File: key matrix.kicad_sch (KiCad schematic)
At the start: 62 parts, among them J3 Conn_01x04_MountingPin, J4 Conn_01x04_MountingPin, SW1 SW_Push, SW10 SW_Push, SW11 SW_Push, SW12 SW_Push, SW13 SW_Push, SW14 SW_Push, SW15 SW_Push, SW16 SW_Push, SW17 SW_Push, SW18 SW_Push, SW19 SW_Push, SW2 SW_Push, SW20 SW_Push, SW21 SW_Push, SW22 SW_Push, SW23 SW_Push, SW24 SW_Push, SW25 SW_Push, SW26 SW_Push, SW27 SW_Push, SW28 SW_Push, SW29 SW_Push, SW3 SW_Push, SW30 SW_Push, SW31 SW_Push, SW32 SW_Push, SW33 SW_Push, SW34 SW_Push, SW35 SW_Push, SW36 SW_Push, SW37 SW_Push, SW38 SW_Push, SW39 SW_Push, SW4 SW_Push, SW40 SW_Push, SW41 SW_Push, SW42 SW_Push, SW43 RotaryEncoder_Switch_MP, SW44 RotaryEncoder_Switch_MP, SW45 SW_Push, SW46 SW_Push, SW47 SW_Push, SW48 SW_Push, SW5 SW_Push, SW6 SW_Push, SW7 SW_Push, SW8 SW_Push, SW9 SW_Push, U1 BAT54CTB6_R1_00001, U10 BAT54CTB6_R1_00001, U11 BAT54CTB6_R1_00001, U12 BAT54CTB6_R1_00001, U2 BAT54CTB6_R1_00001, U3 BAT54CTB6_R1_00001, U4 BAT54CTB6_R1_00001, U5 BAT54CTB6_R1_00001, U6 BAT54CTB6_R1_00001, U7 BAT54CTB6_R1_00001, U8 BAT54CTB6_R1_00001, U9 BAT54CTB6_R1_00001

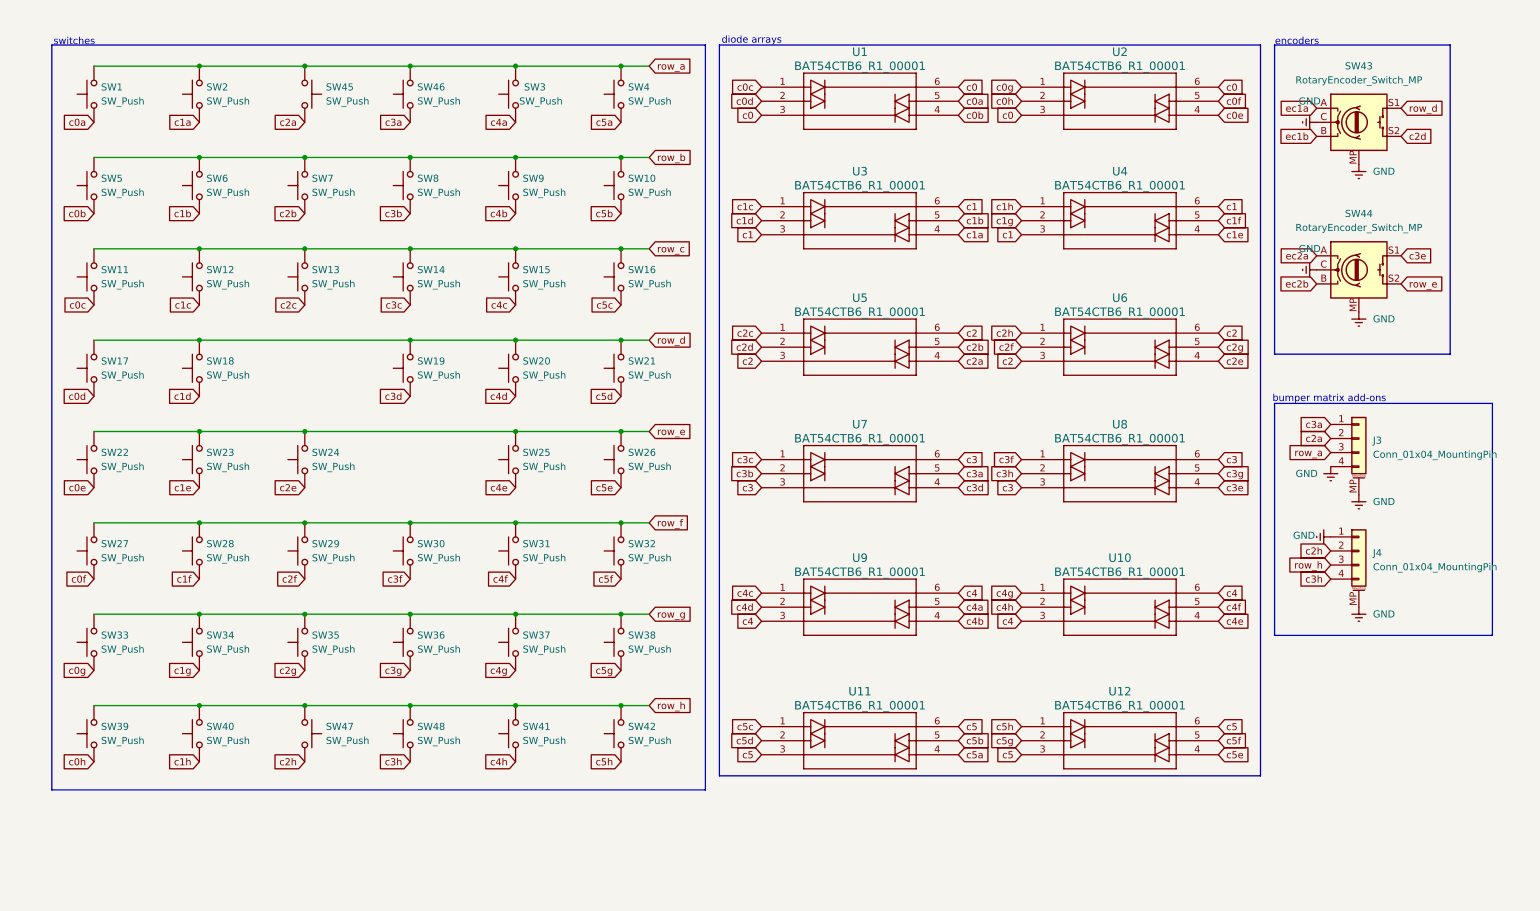
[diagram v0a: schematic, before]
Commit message: parpar v2 RC2
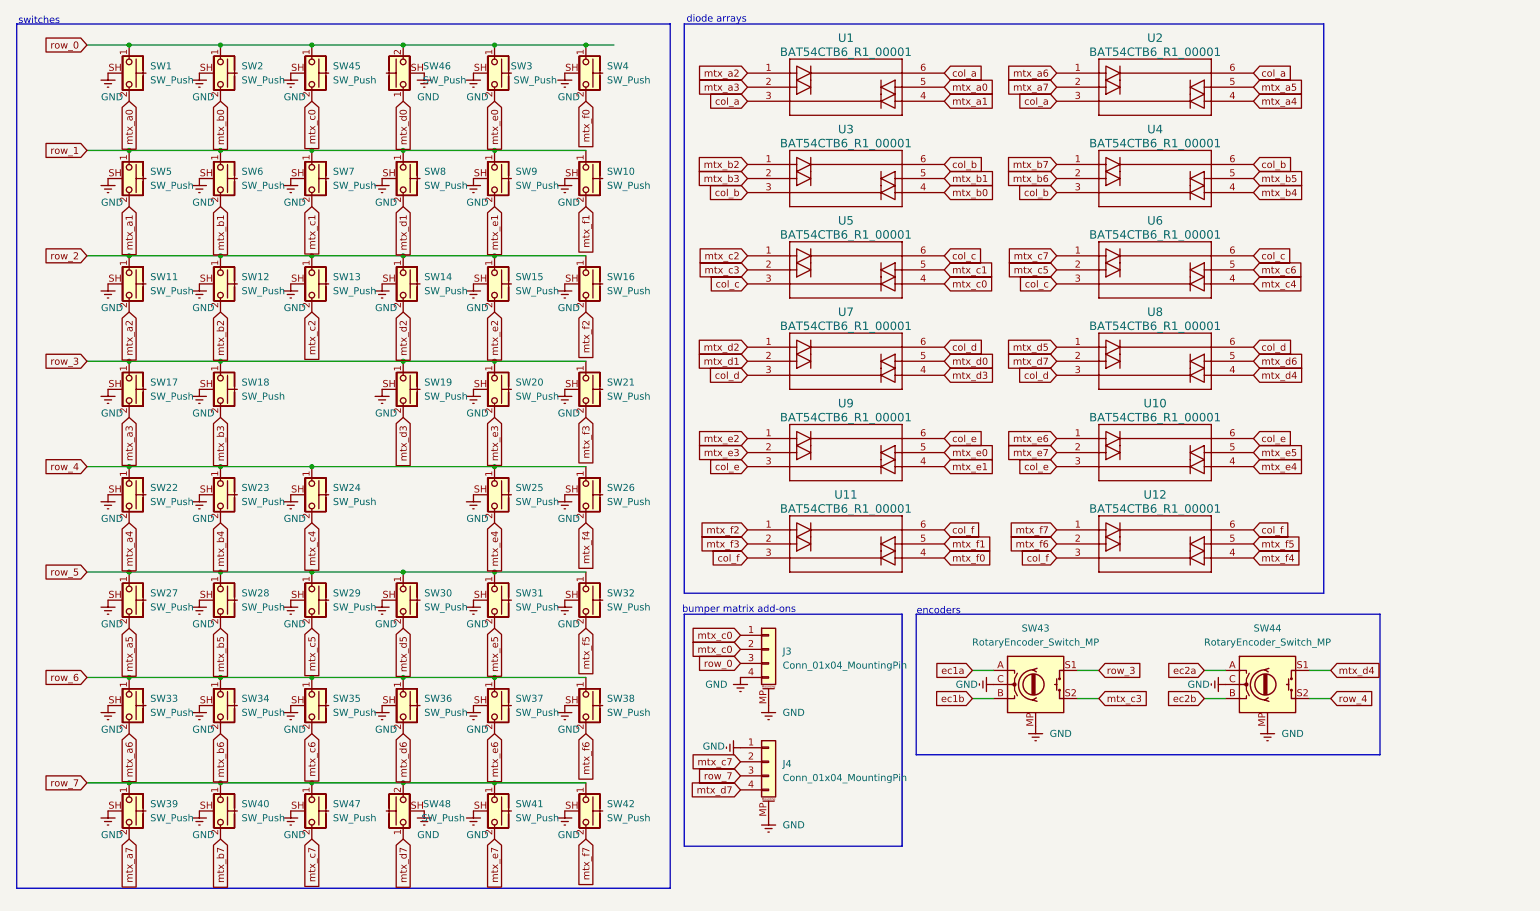
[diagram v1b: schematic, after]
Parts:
- SW1, SW10, SW11, SW12, SW13, SW14, SW15, SW16, SW17, SW18, SW19, SW2, SW20, SW21, SW22, SW23, SW24, SW25, SW26, SW27, SW28, SW29, SW3, SW30, SW31, SW32, SW33, SW34, SW35, SW36, SW37, SW38, SW39, SW4, SW40, SW41, SW42, SW5, SW6, SW7, SW8, SW9: footprint coquette_footprints:choc1u-hs-modded -> coquette_footprints:SW_Hotswap_Kailh_Choc_V1V2_Plated_modded; symbol Switch:SW_Push -> Switch:SW_Push_Shielded
- SW45, SW46, SW47, SW48: symbol Switch:SW_Push -> Switch:SW_Push_Shielded
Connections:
- net GND: now also SW1.SH (B), SW10.SH (B), SW11.SH (B), SW12.SH (B), SW13.SH (B), SW14.SH (B), SW15.SH (B), SW16.SH (B), SW17.SH (B), SW18.SH (B), SW19.SH (B), SW2.SH (B), SW20.SH (B), SW21.SH (B), SW22.SH (B), SW23.SH (B), SW24.SH (B), SW25.SH (B), SW26.SH (B), SW27.SH (B), SW28.SH (B), SW29.SH (B), SW3.SH (B), SW30.SH (B), SW31.SH (B), SW32.SH (B), SW33.SH (B), SW34.SH (B), SW35.SH (B), SW36.SH (B), SW37.SH (B), SW38.SH (B), SW39.SH (B), SW4.SH (B), SW40.SH (B), SW41.SH (B), SW42.SH (B), SW45.SH (B), SW46.SH (B), SW47.SH (B), SW48.SH (B), SW5.SH (B), SW6.SH (B), SW7.SH (B), SW8.SH (B), SW9.SH (B)
- net c0 renamed col_a
- net c0a renamed mtx_a0
- net mtx_a0: now also SW1.2; no longer SW1.1
- net c0b renamed mtx_a1
- net mtx_a1: now also SW5.2; no longer SW5.1
- net c0c renamed mtx_a2
- net mtx_a2: now also SW11.2; no longer SW11.1
- net c0d renamed mtx_a3
- net mtx_a3: now also SW17.2; no longer SW17.1
- net c0e renamed mtx_a4
- net mtx_a4: now also SW22.2; no longer SW22.1
- net c0f renamed mtx_a5
- net mtx_a5: now also SW27.2; no longer SW27.1
- net c0g renamed mtx_a6
- net mtx_a6: now also SW33.2; no longer SW33.1
- net c0h renamed mtx_a7
- net mtx_a7: now also SW39.2; no longer SW39.1
- net c1 renamed col_b
- net c1a renamed mtx_b0
- net mtx_b0: now also SW2.2; no longer SW2.1
- net c1b renamed mtx_b1
- net mtx_b1: now also SW6.2; no longer SW6.1
- net c1c renamed mtx_b2
- net mtx_b2: now also SW12.2; no longer SW12.1
- net c1d renamed mtx_b3
- net mtx_b3: now also SW18.2; no longer SW18.1
- net c1e renamed mtx_b4
- net mtx_b4: now also SW23.2; no longer SW23.1
- net c1f renamed mtx_b5
- net mtx_b5: now also SW28.2; no longer SW28.1
- net c1g renamed mtx_b6
- net mtx_b6: now also SW34.2; no longer SW34.1
- net c1h renamed mtx_b7
- net mtx_b7: now also SW40.2; no longer SW40.1
- net c2 renamed col_c
- net c2a renamed mtx_c0
- net mtx_c0: now also J3.1 (Pin_1)
- net c2b renamed mtx_c1
- net mtx_c1: now also SW7.2; no longer SW7.1
- net c2c renamed mtx_c2
- net mtx_c2: now also SW13.2; no longer SW13.1
- net c2d renamed mtx_c3
- net c2e renamed mtx_c4
- net mtx_c4: now also SW24.2; no longer SW24.1
- net c2f renamed mtx_c5
- net mtx_c5: now also SW29.2; no longer SW29.1
- net c2g renamed mtx_c6
- net mtx_c6: now also SW35.2; no longer SW35.1
- net c2h renamed mtx_c7
- net c3 renamed col_d
- net c3a renamed mtx_d0
- net mtx_d0: no longer J3.1 (Pin_1)
- net c3b renamed mtx_d1
- net mtx_d1: now also SW8.2; no longer SW8.1
- net c3c renamed mtx_d2
- net mtx_d2: now also SW14.2; no longer SW14.1
- net c3d renamed mtx_d3
- net mtx_d3: now also SW19.2; no longer SW19.1
- net c3e renamed mtx_d4
- net c3f renamed mtx_d5
- net mtx_d5: now also SW30.2; no longer SW30.1
- net c3g renamed mtx_d6
- net mtx_d6: now also SW36.2; no longer SW36.1
- net c3h renamed mtx_d7
- net c4 renamed col_e
- net c4a renamed mtx_e0
- net mtx_e0: now also SW3.2; no longer SW3.1
- net c4b renamed mtx_e1
- net mtx_e1: now also SW9.2; no longer SW9.1
- net c4c renamed mtx_e2
- net mtx_e2: now also SW15.2; no longer SW15.1
- net c4d renamed mtx_e3
- net mtx_e3: now also SW20.2; no longer SW20.1
- net c4e renamed mtx_e4
- net mtx_e4: now also SW25.2; no longer SW25.1
- net c4f renamed mtx_e5
- net mtx_e5: now also SW31.2; no longer SW31.1
- net c4g renamed mtx_e6
- net mtx_e6: now also SW37.2; no longer SW37.1
- net c4h renamed mtx_e7
- net mtx_e7: now also SW41.2; no longer SW41.1
- net c5 renamed col_f
- net c5a renamed mtx_f0
- net mtx_f0: now also SW4.2; no longer SW4.1
- net c5b renamed mtx_f1
- net mtx_f1: now also SW10.2; no longer SW10.1
- net c5c renamed mtx_f2
- net mtx_f2: now also SW16.2; no longer SW16.1
- net c5d renamed mtx_f3
- net mtx_f3: now also SW21.2; no longer SW21.1
- net c5e renamed mtx_f4
- net mtx_f4: now also SW26.2; no longer SW26.1
- net c5f renamed mtx_f5
- net mtx_f5: now also SW32.2; no longer SW32.1
- net c5g renamed mtx_f6
- net mtx_f6: now also SW38.2; no longer SW38.1
- net c5h renamed mtx_f7
- net mtx_f7: now also SW42.2; no longer SW42.1
- removed net row_a: J3.3 (Pin_3), SW1.2, SW2.2, SW3.2, SW4.2, SW45.1, SW46.2
- removed net row_b: SW10.2, SW5.2, SW6.2, SW7.2, SW8.2, SW9.2
- removed net row_c: SW11.2, SW12.2, SW13.2, SW14.2, SW15.2, SW16.2
- removed net row_d: SW17.2, SW18.2, SW19.2, SW20.2, SW21.2, SW43.S1
- removed net row_e: SW22.2, SW23.2, SW24.2, SW25.2, SW26.2, SW44.S2
- removed net row_f: SW27.2, SW28.2, SW29.2, SW30.2, SW31.2, SW32.2
- removed net row_g: SW33.2, SW34.2, SW35.2, SW36.2, SW37.2, SW38.2
- removed net row_h: J4.3 (Pin_3), SW39.2, SW40.2, SW41.2, SW42.2, SW47.1, SW48.2
- new net row_0: J3.3 (Pin_3), SW1.1, SW2.1, SW3.1, SW4.1, SW45.1, SW46.2
- new net row_1: SW10.1, SW5.1, SW6.1, SW7.1, SW8.1, SW9.1
- new net row_2: SW11.1, SW12.1, SW13.1, SW14.1, SW15.1, SW16.1
- new net row_3: SW17.1, SW18.1, SW19.1, SW20.1, SW21.1, SW43.S1
- new net row_4: SW22.1, SW23.1, SW24.1, SW25.1, SW26.1, SW44.S2
- new net row_5: SW27.1, SW28.1, SW29.1, SW30.1, SW31.1, SW32.1
- new net row_6: SW33.1, SW34.1, SW35.1, SW36.1, SW37.1, SW38.1
- new net row_7: J4.3 (Pin_3), SW39.1, SW40.1, SW41.1, SW42.1, SW47.1, SW48.2
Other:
- moved on the sheet: J3, J4, SW43, SW44, U1, U10, U11, U12, U2, U3, U4, U5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
